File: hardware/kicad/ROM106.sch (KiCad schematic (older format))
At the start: 55 parts, among them J1 Screw_Terminal_01x03, J2 Screw_Terminal_01x03, J3 CAN, J4 Screw_Terminal_01x03, J5 Screw_Terminal_01x03, J6 Screw_Terminal_01x03, J7 Screw_Terminal_01x03, K1 PE014F05, K2 PE014F05, K3 PE014F05, K4 PE014F05, K5 PE014F05, K6 PE014F05, SW1 INSTANCE, SW2 BUS, SW3 PRG, U1 L293D, U2 MCP2551-I-P, U3 TMR_2411, U4 L293D, U5 L293D, U6 74HC595, U7 Teensy_3.2, U8 MAX6816

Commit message: Refactor
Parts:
- K1, K2, K3, K4, K5, K6: symbol ROM104-rescue:SPDT_RELAY-pdjr-ROM104-rescue -> ROM106-rescue:SPDT_RELAY-pdjr-ROM104-rescue-ROM104-rescue
- U3: symbol ROM104-rescue:TMR_2411-pdjr-ROM104-rescue -> ROM106-rescue:TMR_2411-pdjr-ROM104-rescue-ROM104-rescue
- U7: symbol ROM104-rescue:Teensy_3.2-pdjr-ROM104-rescue -> ROM106-rescue:Teensy_3.2-pdjr-ROM104-rescue-ROM104-rescue
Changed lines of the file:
@@
 NoConn ~ 9100 1850
 $Comp
-L ROM104-rescue:TMR_2411-pdjr-ROM104-rescue U3
+L ROM106-rescue:TMR_2411-pdjr-ROM104-rescue-ROM104-rescue U3
 U 1 1 6327DB22
 P 2950 5050
@@
 ADDR_7
 $Comp
-L ROM104-rescue:Teensy_3.2-pdjr-ROM104-rescue U7
+L ROM106-rescue:Teensy_3.2-pdjr-ROM104-rescue-ROM104-rescue U7
 U 1 1 60F2AB82
 P 10200 3150
@@
 	7050 2700 7300 2700
 $Comp
-L ROM104-rescue:SPDT_RELAY-pdjr-ROM104-rescue K6
+L ROM106-rescue:SPDT_RELAY-pdjr-ROM104-rescue-ROM104-rescue K6
 U 1 1 637805D9
 P 6950 3200
@@
 $EndComp
 $Comp
-L ROM104-rescue:SPDT_RELAY-pdjr-ROM104-rescue K5
+L ROM106-rescue:SPDT_RELAY-pdjr-ROM104-rescue-ROM104-rescue K5
 U 1 1 637805CC
 P 6100 3200
@@
 	5000 3000 5050 3000
 $Comp
-L ROM104-rescue:SPDT_RELAY-pdjr-ROM104-rescue K4
+L ROM106-rescue:SPDT_RELAY-pdjr-ROM104-rescue-ROM104-rescue K4
 U 1 1 63768F03
 P 4700 3200
@@
 $EndComp
 $Comp
-L ROM104-rescue:SPDT_RELAY-pdjr-ROM104-rescue K3
+L ROM106-rescue:SPDT_RELAY-pdjr-ROM104-rescue-ROM104-rescue K3
 U 1 1 63768EF6
 P 3850 3200
@@
 	2750 3000 2800 3000
 $Comp
-L ROM104-rescue:SPDT_RELAY-pdjr-ROM104-rescue K2
+L ROM106-rescue:SPDT_RELAY-pdjr-ROM104-rescue-ROM104-rescue K2
 U 1 1 632D0338
 P 2450 3200
@@
 	2950 2000 3000 2000
 $Comp
-L ROM104-rescue:SPDT_RELAY-pdjr-ROM104-rescue K1
+L ROM106-rescue:SPDT_RELAY-pdjr-ROM104-rescue-ROM104-rescue K1
 U 1 1 632C2C12
 P 1600 3200
@@
 U 1 1 6355CB0C
 P 5850 6500
-F 0 "C10" H 6000 6500 50  0000 C CNN
-F 1 "100nF" H 5650 6500 50  0000 C CNN
+F 0 "C10" V 5900 6400 50  0000 C CNN
+F 1 "100nF" V 5900 6650 50  0000 C CNN
 F 2 "Capacitor_THT:CP_Radial_D5.0mm_P2.00mm" H 5850 6500 50  0001 C CNN
 F 3 "~" H 5850 6500 50  0001 C CNN

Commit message: Redraw PCB
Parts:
- removed C1, C10, C8, C9: 100nF, Capacitor_THT:CP_Radial_D5.0mm_P2.00mm, symbol Device:CP_Small
- removed D1, D2, D3, D4, D5, D6, D7, D8, D9: LED, LED_THT:LED_D1.8mm_W3.3mm_H2.4mm, symbol Device:LED
- removed F1: 1A, Fuse:Fuse_Littelfuse_395Series, symbol Device:Polyfuse
- removed J3: CAN, Connector_PinHeader_2.54mm:PinHeader_1x05_P2.54mm_Vertical, symbol Connector:Screw_Terminal_01x05
- removed R1: 4K7, Resistor_THT:R_Axial_DIN0207_L6.3mm_D2.5mm_P2.54mm_Vertical, symbol Device:R
- removed R10, R11, R3, R4, R5, R6, R7, R8, R9: 470R, Resistor_THT:R_Axial_DIN0207_L6.3mm_D2.5mm_P2.54mm_Vertical, symbol Device:R
- removed R2: 120R, Resistor_THT:R_Axial_DIN0207_L6.3mm_D2.5mm_P7.62mm_Horizontal, symbol Device:R
- removed SW1: INSTANCE, Package_DIP:DIP-16_W7.62mm, symbol Switch:SW_DIP_x08
- removed SW2: BUS, Package_DIP:DIP-4_W7.62mm_LongPads, symbol Switch:SW_DIP_x02
- removed SW3: PRG, PDJR-connectors:PCB_PUSH_BUTTON, symbol Switch:SW_Push
- removed U2: MCP2551-I-P, Package_DIP:DIP-8_W7.62mm, symbol Interface_CAN_LIN:MCP2551-I-P
- removed U3: TMR_2411, PDJR_DC-DC_Converters:TMR_2411, symbol ROM106-rescue:TMR_2411-pdjr-ROM104-rescue-ROM104-rescue
- removed U6: 74HC595, Package_DIP:DIP-16_W7.62mm_Socket_LongPads, symbol 74xx:74HC595
- removed U7: Teensy_3.2, Package_DIP:DIP-28_W15.24mm_LongPads, symbol ROM106-rescue:Teensy_3.2-pdjr-ROM104-rescue-ROM104-rescue
- removed U8: MAX6816, Package_TO_SOT_SMD:SOT-143, symbol Interface:MAX6816
- renumbered J1 to J10, J2 to J11, J4 to J12, J5 to J13, J6 to J14, J7 to J15
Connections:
- net labels added: D20, D21, D22, D23, D5, D6, D8, D9
- net labels removed: ADDR_0, ADDR_1, ADDR_2, ADDR_3, ADDR_4, ADDR_5, ADDR_6, ADDR_7, CAN_H, CAN_L, CAN_RX, CAN_SCR, CAN_TX, CH1_EN, CH2_EN, CH3_EN, CH4_EN, CH5_EN, CH6_EN, LED_PWR, MPX_CLOCK, MPX_DATA, MPX_LATCH, NET_C, PRG, RST, SET, TERM_A, TERM_B, TRANSMIT_LED
- wire segments 346 -> 201
- no-connect marks 7 -> 0
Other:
- note removed: "CONFIGURATION"
- note removed: "DISPLAY"
- note removed: "POWER SUPPLY & CAN INTERFACE"
- note removed: "RELAY OUTPUTS"
- moved on the sheet: C2, C3, C4, C5, C6, C7, J10, J11, J12, J13, J14, J15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

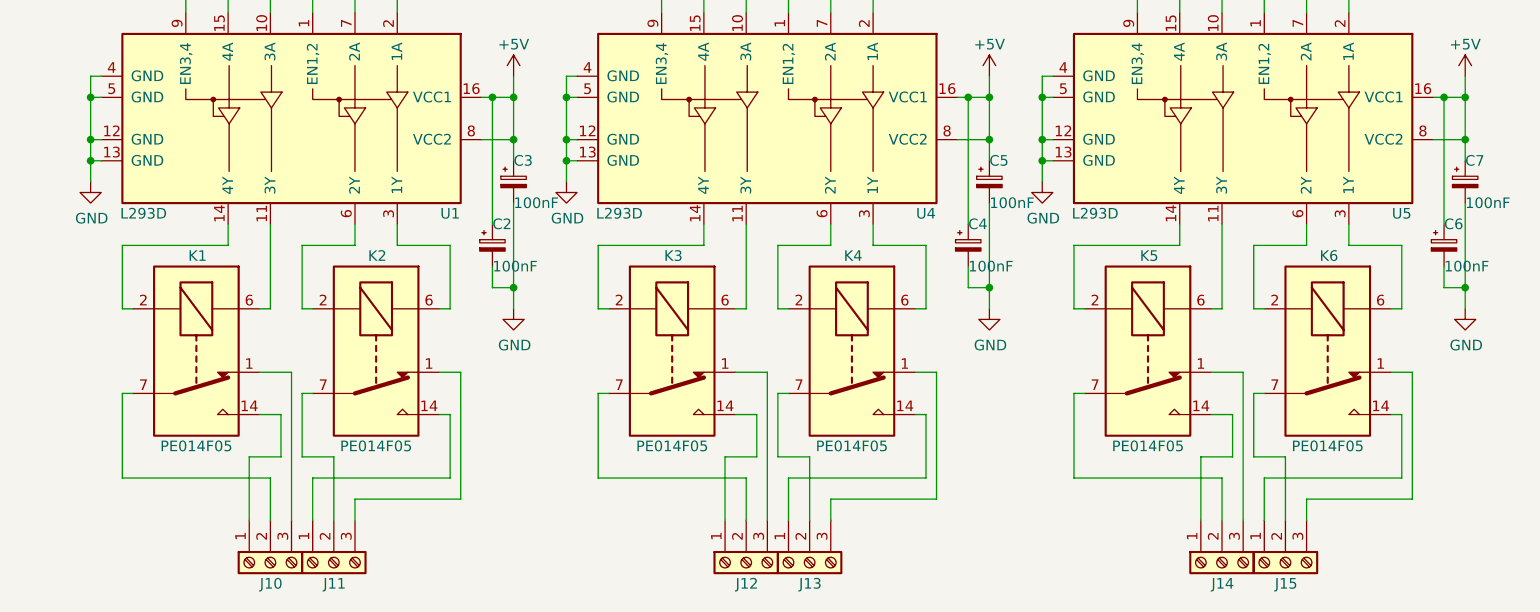
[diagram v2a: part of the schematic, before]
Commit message: Tweak
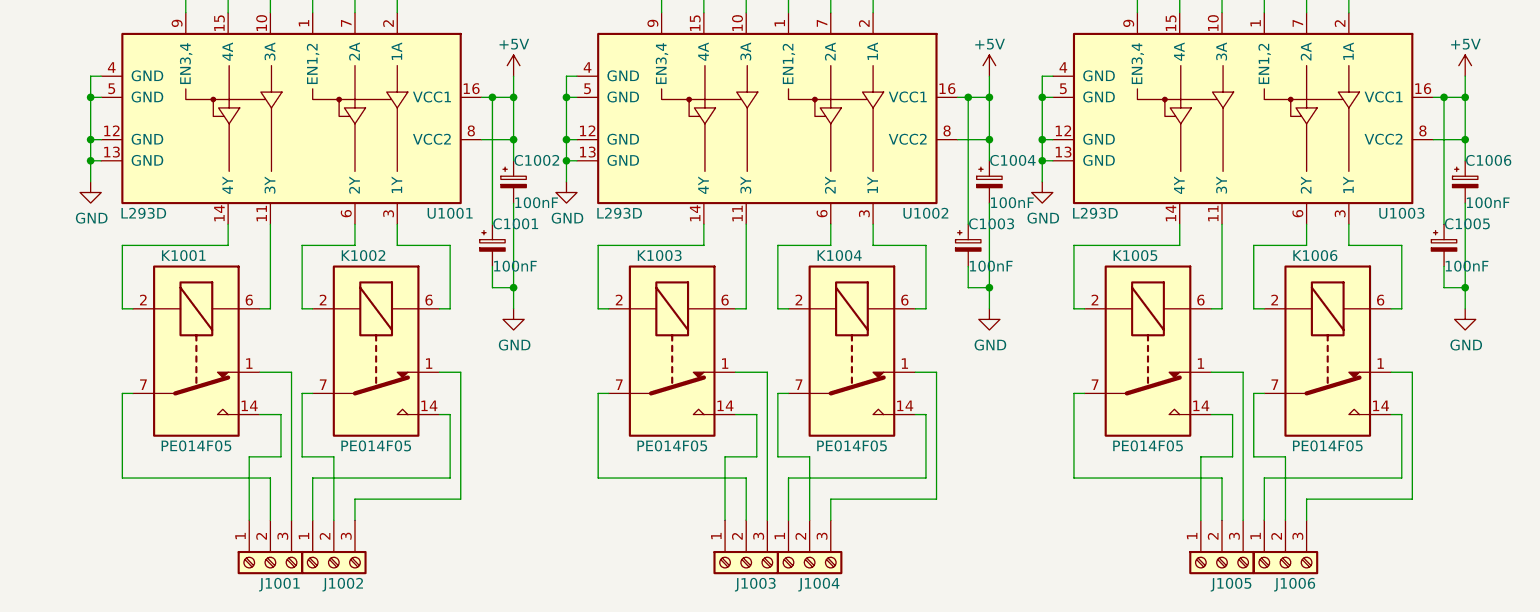
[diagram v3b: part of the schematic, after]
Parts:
- renumbered C2 to C1001, C3 to C1002, C4 to C1003, C5 to C1004, C6 to C1005, C7 to C1006, J10 to J1001, J11 to J1002, J12 to J1003, J13 to J1004, J14 to J1005, J15 to J1006, K1 to K1001, K2 to K1002, K3 to K1003, K4 to K1004, K5 to K1005, K6 to K1006, U1 to U1001, U4 to U1002, U5 to U1003
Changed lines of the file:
@@
 	9000 3400 9000 3300
 $Comp
-L Device:CP_Small C6
+L Device:CP_Small C1005
 U 1 1 63765276
 P 9000 3200
-F 0 "C6" H 9000 3300 50  0000 L CNN
+F 0 "C1005" H 9000 3300 50  0000 L CNN
 F 1 "100nF" H 9000 3100 50  0000 L CNN
 F 2 "Capacitor_THT:CP_Radial_D5.0mm_P2.00mm" H 9000 3200 50  0001 C CNN
@@
 $EndComp
 $Comp
-L Device:CP_Small C7
+L Device:CP_Small C1006
 U 1 1 63765270
 P 9100 2900
-F 0 "C7" H 9100 3000 50  0000 L CNN
+F 0 "C1006" H 9100 3000 50  0000 L CNN
 F 1 "100nF" H 9100 2800 50  0000 L CNN
 F 2 "Capacitor_THT:CP_Radial_D5.0mm_P2.00mm" H 9100 2900 50  0001 C CNN
@@
 $EndComp
 $Comp
-L power:GND #PWR014
+L power:GND #PWR01009
 U 1 1 6376526A
 P 9100 3500
-F 0 "#PWR014" H 9100 3250 50  0001 C CNN
+F 0 "#PWR01009" H 9100 3250 50  0001 C CNN
 F 1 "GND" H 9105 3327 50  0000 C CNN
 F 2 "" H 9100 3500 50  0001 C CNN
@@
 	8950 2500 9000 2500
 $Comp
-L power:+5V #PWR013
+L power:+5V #PWR01008
 U 1 1 63765256
 P 9100 2400
-F 0 "#PWR013" H 9100 2250 50  0001 C CNN
+F 0 "#PWR01008" H 9100 2250 50  0001 C CNN
 F 1 "+5V" H 9100 2550 50  0000 C CNN
 F 2 "" H 9100 2400 50  0001 C CNN
@@
 	6750 3400 6750 3300
 $Comp
-L Device:CP_Small C4
+L Device:CP_Small C1003
 U 1 1 63748987
 P 6750 3200
-F 0 "C4" H 6750 3300 50  0000 L CNN
+F 0 "C1003" H 6750 3300 50  0000 L CNN
 F 1 "100nF" H 6750 3100 50  0000 L CNN
 F 2 "Capacitor_THT:CP_Radial_D5.0mm_P2.00mm" H 6750 3200 50  0001 C CNN
@@
 $EndComp
 $Comp
-L Device:CP_Small C5
+L Device:CP_Small C1004
 U 1 1 63748981
 P 6850 2900
-F 0 "C5" H 6850 3000 50  0000 L CNN
+F 0 "C1004" H 6850 3000 50  0000 L CNN
 F 1 "100nF" H 6850 2800 50  0000 L CNN
 F 2 "Capacitor_THT:CP_Radial_D5.0mm_P2.00mm" H 6850 2900 50  0001 C CNN
@@
 $EndComp
 $Comp
-L power:GND #PWR010
+L power:GND #PWR01006
 U 1 1 6374897B
 P 6850 3500
-F 0 "#PWR010" H 6850 3250 50  0001 C CNN
+F 0 "#PWR01006" H 6850 3250 50  0001 C CNN
 F 1 "GND" H 6855 3327 50  0000 C CNN
 F 2 "" H 6850 3500 50  0001 C CNN
@@
 	6700 2500 6750 2500
 $Comp
-L power:+5V #PWR09
+L power:+5V #PWR01005
 U 1 1 63748967
 P 6850 2400
-F 0 "#PWR09" H 6850 2250 50  0001 C CNN
+F 0 "#PWR01005" H 6850 2250 50  0001 C CNN
 F 1 "+5V" H 6850 2550 50  0000 C CNN
 F 2 "" H 6850 2400 50  0001 C CNN
@@
 	4500 3400 4500 3300
 $Comp
-L Device:CP_Small C2
+L Device:CP_Small C1001
 U 1 1 6352B944
 P 4500 3200
-F 0 "C2" H 4500 3300 50  0000 L CNN
+F 0 "C1001" H 4500 3300 50  0000 L CNN
 F 1 "100nF" H 4500 3100 50  0000 L CNN
 F 2 "Capacitor_THT:CP_Radial_D5.0mm_P2.00mm" H 4500 3200 50  0001 C CNN
@@
 $EndComp
 $Comp
-L Device:CP_Small C3
+L Device:CP_Small C1002
 U 1 1 63524B62
 P 4600 2900
-F 0 "C3" H 4600 3000 50  0000 L CNN
+F 0 "C1002" H 4600 3000 50  0000 L CNN
 F 1 "100nF" H 4600 2800 50  0000 L CNN
 F 2 "Capacitor_THT:CP_Radial_D5.0mm_P2.00mm" H 4600 2900 50  0001 C CNN
@@
 Connection ~ 4050 1900
 $Comp
-L power:GND #PWR07
+L power:GND #PWR01003
 U 1 1 63471B52
 P 4600 3500
-F 0 "#PWR07" H 4600 3250 50  0001 C CNN
+F 0 "#PWR01003" H 4600 3250 50  0001 C CNN
 F 1 "GND" H 4605 3327 50  0000 C CNN
 F 2 "" H 4600 3500 50  0001 C CNN
@@
 	7100 2800 7100 2900
 $Comp
-L power:GND #PWR012
+L power:GND #PWR01007
 U 1 1 63780608
 P 7100 2900
-F 0 "#PWR012" H 7100 2650 50  0001 C CNN
+F 0 "#PWR01007" H 7100 2650 50  0001 C CNN
 F 1 "GND" H 7105 2727 50  0000 C CNN
 F 2 "" H 7100 2900 50  0001 C CNN
@@
 	8550 3200 8800 3200
 $Comp
-L ROM106-rescue:SPDT_RELAY-pdjr-ROM104-rescue-ROM104-rescue K6
+L ROM106-rescue:SPDT_RELAY-pdjr-ROM104-rescue-ROM104-rescue K1006
 U 1 1 637805D9
 P 8450 3700
-F 0 "K6" V 8000 3750 50  0000 R CNN
+F 0 "K1006" V 8000 3750 50  0000 R CNN
 F 1 "PE014F05" V 8900 3700 50  0000 C CNN
 F 2 "PDJR_Relays:PE014F05" H 8900 3650 50  0001 L CNN
@@
 $EndComp
 $Comp
-L ROM106-rescue:SPDT_RELAY-pdjr-ROM104-rescue-ROM104-rescue K5
+L ROM106-rescue:SPDT_RELAY-pdjr-ROM104-rescue-ROM104-rescue K1005
 U 1 1 637805CC
 P 7600 3700
-F 0 "K5" V 7150 3750 50  0000 R CNN
+F 0 "K1005" V 7150 3750 50  0000 R CNN
 F 1 "PE014F05" V 8050 3700 50  0000 C CNN
 F 2 "PDJR_Relays:PE014F05" H 8050 3650 50  0001 L CNN
@@
 	8050 4500 8050 3800
 $Comp
-L Driver_Motor:L293D U5
+L Driver_Motor:L293D U1003
 U 1 1 637805AC
 P 7950 2600
-F 0 "U5" V 8400 3450 50  0000 C CNN
+F 0 "U1003" V 8400 3450 50  0000 C CNN
 F 1 "L293D" V 8400 2000 50  0000 C CNN
 F 2 "Package_DIP:DIP-16_W7.62mm" H 8200 1850 50  0001 L CNN
@@
 	4850 2700 4900 2700
 $Comp
-L power:GND #PWR08
+L power:GND #PWR01004
 U 1 1 63768F32
 P 4850 2900
-F 0 "#PWR08" H 4850 2650 50  0001 C CNN
+F 0 "#PWR01004" H 4850 2650 50  0001 C CNN
 F 1 "GND" H 4855 2727 50  0000 C CNN
 F 2 "" H 4850 2900 50  0001 C CNN
@@
 	6500 3500 6550 3500
 $Comp
-L ROM106-rescue:SPDT_RELAY-pdjr-ROM104-rescue-ROM104-rescue K4
+L ROM106-rescue:SPDT_RELAY-pdjr-ROM104-rescue-ROM104-rescue K1004
 U 1 1 63768F03
 P 6200 3700
-F 0 "K4" V 5750 3750 50  0000 R CNN
+F 0 "K1004" V 5750 3750 50  0000 R CNN
 F 1 "PE014F05" V 6650 3700 50  0000 C CNN
 F 2 "PDJR_Relays:PE014F05" H 6650 3650 50  0001 L CNN
@@
 $EndComp
 $Comp
-L ROM106-rescue:SPDT_RELAY-pdjr-ROM104-rescue-ROM104-rescue K3
+L ROM106-rescue:SPDT_RELAY-pdjr-ROM104-rescue-ROM104-rescue K1003
 U 1 1 63768EF6
 P 5350 3700
-F 0 "K3" V 4900 3750 50  0000 R CNN
+F 0 "K1003" V 4900 3750 50  0000 R CNN
 F 1 "PE014F05" V 5800 3700 50  0000 C CNN
 F 2 "PDJR_Relays:PE014F05" H 5800 3650 50  0001 L CNN
@@
 	6500 3800 6600 3800
 $Comp
-L Driver_Motor:L293D U4
+L Driver_Motor:L293D U1002
 U 1 1 63768ED6
 P 5700 2600
-F 0 "U4" V 6150 3450 50  0000 C CNN
+F 0 "U1002" V 6150 3450 50  0000 C CNN
 F 1 "L293D" V 6150 2000 50  0000 C CNN
 F 2 "Package_DIP:DIP-16_W7.62mm" H 5950 1850 50  0001 L CNN
@@
 	2600 2700 2650 2700
 $Comp
-L power:GND #PWR05
+L power:GND #PWR01001
 U 1 1 636F6993
 P 2600 2900
-F 0 "#PWR05" H 2600 2650 50  0001 C CNN
+F 0 "#PWR01001" H 2600 2650 50  0001 C CNN
 F 1 "GND" H 2605 2727 50  0000 C CNN
 F 2 "" H 2600 2900 50  0001 C CNN
@@
 	4250 3500 4300 3500
 $Comp
-L ROM106-rescue:SPDT_RELAY-pdjr-ROM104-rescue-ROM104-rescue K2
+L ROM106-rescue:SPDT_RELAY-pdjr-ROM104-rescue-ROM104-rescue K1002
 U 1 1 632D0338
 P 3950 3700
-F 0 "K2" V 3500 3750 50  0000 R CNN
+F 0 "K1002" V 3500 3750 50  0000 R CNN
 F 1 "PE014F05" V 4400 3700 50  0000 C CNN
 F 2 "PDJR_Relays:PE014F05" H 4400 3650 50  0001 L CNN
@@
 	4450 2500 4500 2500
 $Comp
-L ROM106-rescue:SPDT_RELAY-pdjr-ROM104-rescue-ROM104-rescue K1
+L ROM106-rescue:SPDT_RELAY-pdjr-ROM104-rescue-ROM104-rescue K1001
 U 1 1 632C2C12
 P 3100 3700
-F 0 "K1" V 2650 3750 50  0000 R CNN
+F 0 "K1001" V 2650 3750 50  0000 R CNN
 F 1 "PE014F05" V 3550 3700 50  0000 C CNN
 F 2 "PDJR_Relays:PE014F05" H 3550 3650 50  0001 L CNN
@@
 	3250 2100 3250 2000
 $Comp
-L power:+5V #PWR06
+L power:+5V #PWR01002
 U 1 1 634BDEB3
 P 4600 2400
-F 0 "#PWR06" H 4600 2250 50  0001 C CNN
+F 0 "#PWR01002" H 4600 2250 50  0001 C CNN
 F 1 "+5V" H 4600 2550 50  0000 C CNN
 F 2 "" H 4600 2400 50  0001 C CNN
@@
 	4250 3800 4350 3800
 $Comp
-L Driver_Motor:L293D U1
+L Driver_Motor:L293D U1001
 U 1 1 631FC180
 P 3450 2600
-F 0 "U1" V 3900 3450 50  0000 C CNN
+F 0 "U1001" V 3900 3450 50  0000 C CNN
 F 1 "L293D" V 3900 2000 50  0000 C CNN
 F 2 "Package_DIP:DIP-16_W7.62mm" H 3700 1850 50  0001 L CNN
@@
 $EndComp
 $Comp
-L Connector:Screw_Terminal_01x03 J10
+L Connector:Screw_Terminal_01x03 J1001
 U 1 1 6369F8B1
 P 3450 4700
-F 0 "J10" V 3550 4750 50  0000 R CNN
+F 0 "J1001" V 3550 4750 50  0000 R CNN
 F 1 "Screw_Terminal_01x03" V 3413 4512 50  0001 R CNN
 F 2 "PDJR_Connectors:8971187_3_PIN_5MM_PLUGGABLE_HEADER" H 3450 4700 50  0001 C CNN
@@
 $EndComp
 $Comp
-L Connector:Screw_Terminal_01x03 J11
+L Connector:Screw_Terminal_01x03 J1002
 U 1 1 636A224A
 P 3750 4700
-F 0 "J11" V 3850 4750 50  0000 R CNN
+F 0 "J1002" V 3850 4750 50  0000 R CNN
 F 1 "Screw_Terminal_01x03" V 3713 4512 50  0001 R CNN
 F 2 "PDJR_Connectors:8971187_3_PIN_5MM_PLUGGABLE_HEADER" H 3750 4700 50  0001 C CNN
@@
 $EndComp
 $Comp
-L Connector:Screw_Terminal_01x03 J12
+L Connector:Screw_Terminal_01x03 J1003
 U 1 1 636A2D0F
 P 5700 4700
-F 0 "J12" V 5800 4750 50  0000 R CNN
+F 0 "J1003" V 5800 4750 50  0000 R CNN
 F 1 "Screw_Terminal_01x03" V 5663 4512 50  0001 R CNN
 F 2 "PDJR_Connectors:8971187_3_PIN_5MM_PLUGGABLE_HEADER" H 5700 4700 50  0001 C CNN
@@
 $EndComp
 $Comp
-L Connector:Screw_Terminal_01x03 J13
+L Connector:Screw_Terminal_01x03 J1004
 U 1 1 636A484F
 P 6000 4700
-F 0 "J13" V 6100 4750 50  0000 R CNN
+F 0 "J1004" V 6100 4750 50  0000 R CNN
 F 1 "Screw_Terminal_01x03" V 5963 4512 50  0001 R CNN
 F 2 "PDJR_Connectors:8971187_3_PIN_5MM_PLUGGABLE_HEADER" H 6000 4700 50  0001 C CNN
@@
 $EndComp
 $Comp
-L Connector:Screw_Terminal_01x03 J14
+L Connector:Screw_Terminal_01x03 J1005
 U 1 1 636A5787
 P 7950 4700
-F 0 "J14" V 8050 4750 50  0000 R CNN
+F 0 "J1005" V 8050 4750 50  0000 R CNN
 F 1 "Screw_Terminal_01x03" V 7913 4512 50  0001 R CNN
 F 2 "PDJR_Connectors:8971187_3_PIN_5MM_PLUGGABLE_HEADER" H 7950 4700 50  0001 C CNN
@@
 $EndComp
 $Comp
-L Connector:Screw_Terminal_01x03 J15
+L Connector:Screw_Terminal_01x03 J1006
 U 1 1 636A695C
 P 8250 4700
-F 0 "J15" V 8350 4750 50  0000 R CNN
+F 0 "J1006" V 8350 4750 50  0000 R CNN
 F 1 "Screw_Terminal_01x03" V 8213 4512 50  0001 R CNN
 F 2 "PDJR_Connectors:8971187_3_PIN_5MM_PLUGGABLE_HEADER" H 8250 4700 50  0001 C CNN
